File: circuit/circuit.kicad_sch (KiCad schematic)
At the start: 22 parts, among them J1 Micro_SD_Card, J2 VGA, J3 USB-C Power, U1 Pico, U2 Z80CPU, U3 AS6C4008-55PCN, U4 TXS0108EPW, U5 TXS0108EPW, U6 TXS0108EPW, U7 74LS393, X1 10Mhz

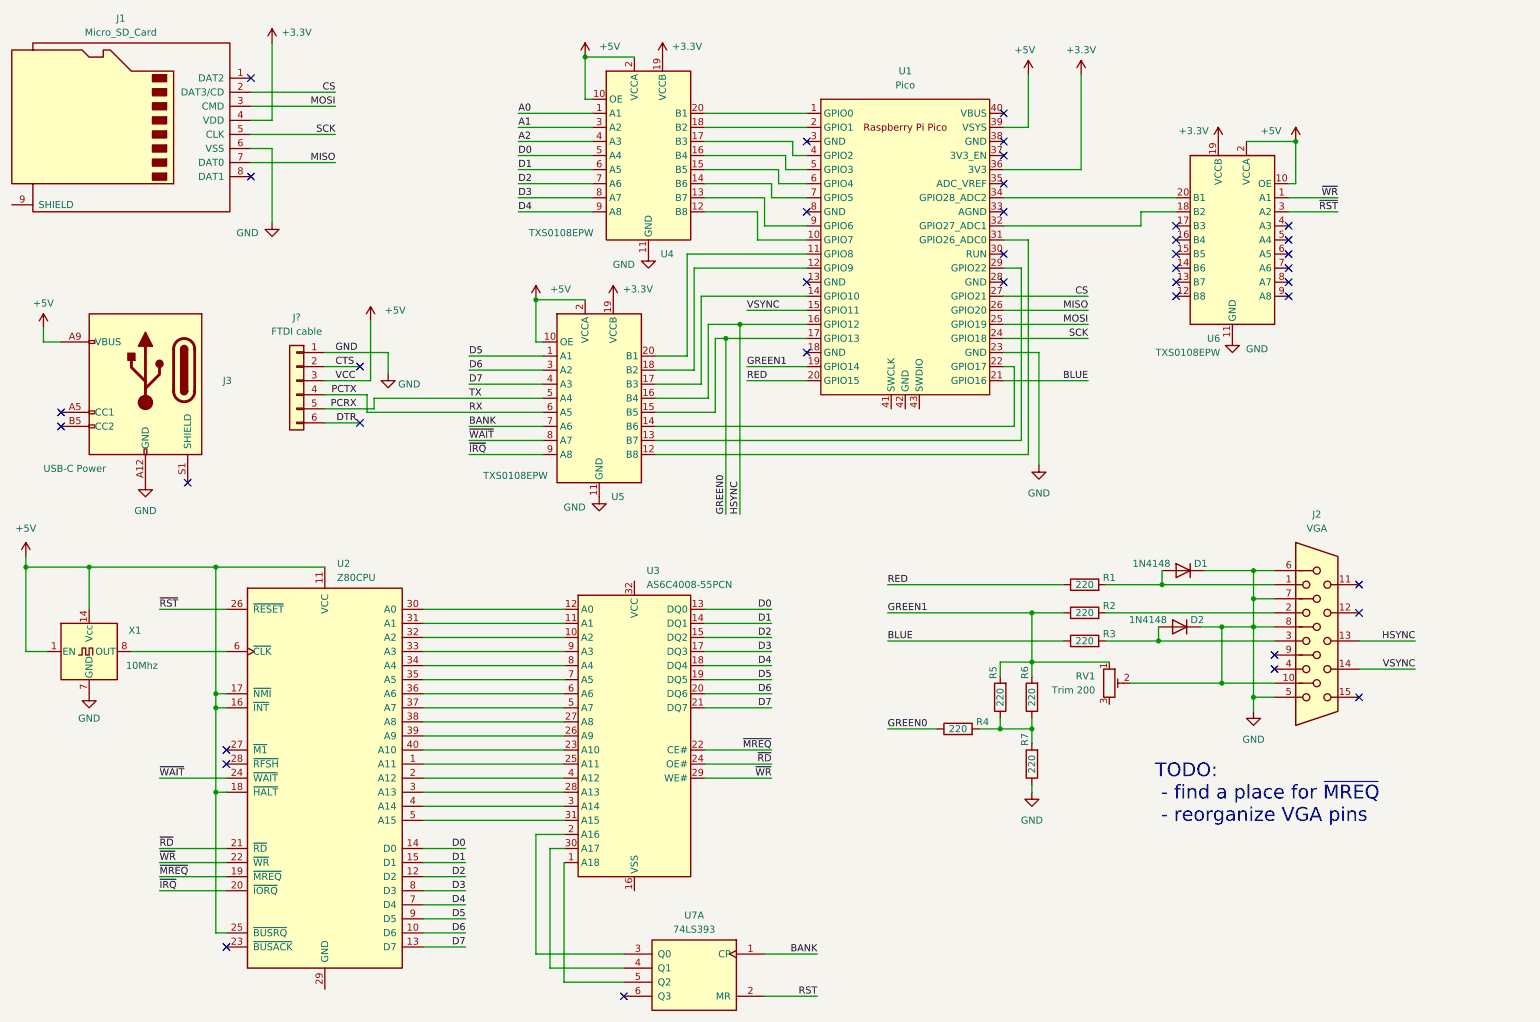
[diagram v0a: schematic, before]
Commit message: .
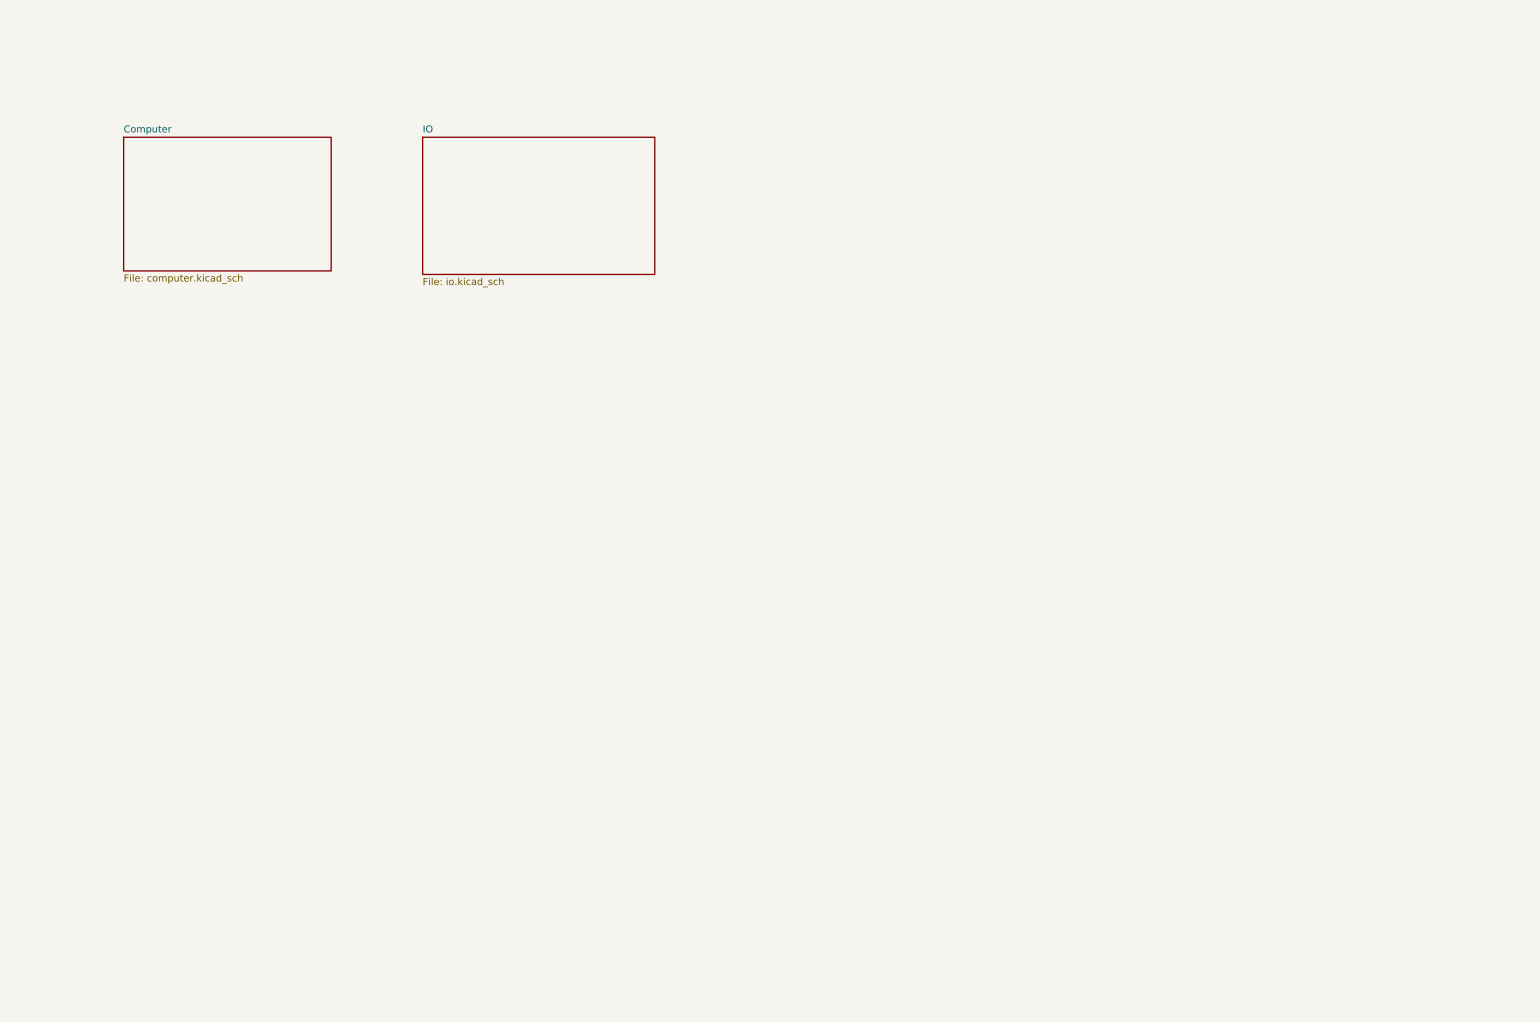
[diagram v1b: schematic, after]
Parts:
- removed D1, D2: 1N4148, Diode_THT:D_DO-35_SOD27_P7.62mm_Horizontal, symbol Diode:1N4148
- removed J1: Micro_SD_Card, symbol Connector:Micro_SD_Card
- removed J2: VGA, symbol Connector:DE15_Receptacle_HighDensity
- removed J3: USB-C Power, symbol Connector:USB_C_Receptacle_PowerOnly_6P
- removed J?: FTDI cable, symbol Connector_Generic:Conn_01x06
- removed R1, R2, R3, R4, R5, R6, R7: 220, symbol Device:R
- removed RV1: Trim 200, symbol Device:R_Potentiometer_Trim
- removed U1: Pico, RPi_Pico:RPi_Pico_SMD_TH, symbol MCU_RaspberryPi_and_Boards:Pico
- removed U2: Z80CPU, symbol CPU:Z80CPU
- removed U3: AS6C4008-55PCN, Package_DIP:DIP-32_W15.24mm, symbol Memory_RAM:AS6C4008-55PCN
- removed U4, U5, U6: TXS0108EPW, Package_SO:TSSOP-20_4.4x6.5mm_P0.65mm, symbol Logic_LevelTranslator:TXS0108EPW
- removed U7: 74LS393, symbol 74xx:74LS393
- removed X1: 10Mhz, Oscillator:Oscillator_DIP-14, symbol Oscillator:CXO_DIP14
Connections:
- no-connect marks 39 -> 0
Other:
- added sheet Computer (computer.kicad_sch)
- added sheet IO (io.kicad_sch)
- note removed: "TODO: - find a place for ~{MREQ} - reorganize VGA pins"
